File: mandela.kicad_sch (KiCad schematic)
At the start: 2 parts

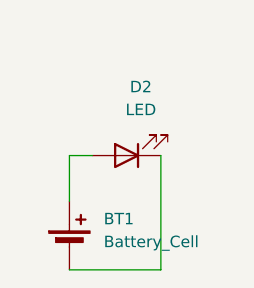
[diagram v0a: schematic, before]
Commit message: Update files
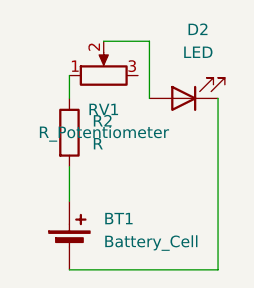
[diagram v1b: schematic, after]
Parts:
- added R2: R, no_silk:R_Axial_DIN0207_L6.3mm_D2.5mm_P7.62mm_Horizontal, symbol Device:R
- added RV1: R_Potentiometer, no_silk:Potentiometer_Vishay_T73YP_Vertical, symbol Device:R_Potentiometer
- D2: footprint LED_THT:LED_D5.0mm -> no_silk:LED_D5.0mm
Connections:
- net at BT1.1 (+): now also R2.2; no longer D2.2 (A)
- new net: D2.2 (A), RV1.2
- new net: R2.1, RV1.1
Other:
- moved on the sheet: D2
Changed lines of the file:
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@@
 	(wire
 		(pts
-			(xy 62.23 104.14) (xy 62.23 99.06)
-		)
-		(stroke
-			(width 0)
-			(type default)
-		)
-	)
-	(wire
-		(pts
-			(xy 72.39 111.76) (xy 62.23 111.76)
-		)
-		(stroke
-			(width 0)
-			(type default)
-		)
-	)
-	(wire
-		(pts
-			(xy 72.39 99.06) (xy 72.39 111.76)
-		)
-		(stroke
-			(width 0)
-			(type default)
-		)
-	)
-	(wire
-		(pts
-			(xy 62.23 99.06) (xy 64.77 99.06)
+			(xy 66.04 86.36) (xy 71.12 86.36)
+		)
+		(stroke
+			(width 0)
+			(type default)
+		)
+	)
+	(wire
+		(pts
+			(xy 62.23 100.33) (xy 62.23 104.14)
+		)
+		(stroke
+			(width 0)
+			(type default)
+		)
+	)
+	(wire
+		(pts
+			(xy 78.74 111.76) (xy 62.23 111.76)
+		)
+		(stroke
+			(width 0)
+			(type default)
+		)
+	)
+	(wire
+		(pts
+			(xy 71.12 86.36) (xy 71.12 92.71)
+		)
+		(stroke
+			(width 0)
+			(type default)
+		)
+	)
+	(wire
+		(pts
+			(xy 62.23 90.17) (xy 62.23 92.71)
+		)
+		(stroke
+			(width 0)
+			(type default)
+		)
+	)
+	(wire
+		(pts
+			(xy 78.74 92.71) (xy 78.74 111.76)
 		)
 		(stroke
@@
 	(symbol
 		(lib_id "Device:LED")
-		(at 68.58 99.06 180)
+		(at 74.93 92.71 180)
 		(unit 1)
 		(exclude_from_sim no)
@@
 		(fields_autoplaced yes)
 		(property "Reference" "D2"
-			(at 70.1675 91.44 0)
+			(at 76.5175 85.09 0)
 			(effects
 				(font
@@
 		)
 		(property "Value" "LED"
-			(at 70.1675 93.98 0)
-			(effects
-				(font
-					(size 1.27 1.27)
-				)
-			)
-		)
-		(property "Footprint" "LED_THT:LED_D5.0mm"
-			(at 68.58 99.06 0)
+			(at 76.5175 87.63 0)
+			(effects
+				(font
+					(size 1.27 1.27)
+				)
+			)
+		)
+		(property "Footprint" "no_silk:LED_D5.0mm"
+			(at 74.93 92.71 0)
 			(effects
 				(font
@@
 		)
 		(property "Datasheet" "~"
-			(at 68.58 99.06 0)
+			(at 74.93 92.71 0)
 			(effects
 				(font
@@
 		)
 		(property "Description" "Light emitting diode"
-			(at 68.58 99.06 0)
+			(at 74.93 92.71 0)
 			(effects
 				(font
@@
 		)
 		(property "Sim.Pins" "1=K 2=A"
-			(at 68.58 99.06 0)
+			(at 74.93 92.71 0)
 			(effects
 				(font
@@
 					(unit 1)
 				)
+			)
+		)
+	)
+	(symbol
+		(lib_id "Device:R")
+		(at 62.23 96.52 0)
+		(unit 1)
+		(exclude_from_sim no)
+		(in_bom yes)
+		(on_board yes)
+		(dnp no)
+		(property "Reference" "R2"
+			(at 64.77 95.2499 0)
+			(effects
+				(font
+					(size 1.27 1.27)
+				)
+				(justify left)
+			)
+		)
+		(property "Value" "R"
+			(at 64.77 97.7899 0)
+			(effects
+				(font
+					(size 1.27 1.27)
+				)
+				(justify left)
+			)
+		)
+		(property "Footprint" "no_silk:R_Axial_DIN0207_L6.3mm_D2.5mm_P7.62mm_Horizontal"
+			(at 60.452 96.52 90)
+			(effects
+				(font
+					(size 1.27 1.27)
+				)
+				(hide yes)
+			)
+		)
+		(property "Datasheet" "~"
+			(at 62.23 96.52 0)
+			(effects
+				(font
+					(size 1.27 1.27)
+				)
+				(hide yes)
+			)
+		)
+		(property "Description" "Resistor"
+			(at 62.23 96.52 0)
+			(effects
+				(font
+					(size 1.27 1.27)
+				)
+				(hide yes)
+			)
+		)
+		(pin "2"
+		)
+		(pin "1"
+		)
+		(instances
+			(project ""
+				(path "/6e1b4b5d-1e46-4a59-af59-5db0f65b54fa"
+					(reference "R2")
+					(unit 1)
+				)
+			)
+		)
+	)
+	(symbol
+		(lib_id "Device:R_Potentiometer")
+		(at 66.04 90.17 90)
+		(unit 1)
+		(exclude_from_sim no)
+		(in_bom yes)
+		(on_board yes)
+		(dnp no)
+		(fields_autoplaced yes)
+		(property "Reference" "RV1"
+			(at 66.04 93.98 90)
+			(effects
+				(font
+					(size 1.27 1.27)
+				)
+			)
+		)
+		(property "Value" "R_Potentiometer"
+			(at 66.04 96.52 90)
+			(effects
+				(font
+					(size 1.27 1.27)
+				)
+			)
+		)
+		(property "Footprint" "no_silk:Potentiometer_Vishay_T73YP_Vertical"
+			(at 66.04 90.17 0)
+			(effects
+				(font
+					(size 1.27 1.27)
+				)
+				(hide yes)
+			)
+		)
+		(property "Datasheet" "~"
+			(at 66.04 90.17 0)
+			(effects
+				(font
+					(size 1.27 1.27)
+				)
+				(hide yes)
+			)
+		)
+		(property "Description" "Potentiometer"
+			(at 66.04 90.17 0)
+			(effects
+				(font
+					(size 1.27 1.27)
+				)
+				(hide yes)
+			)
+		)
+		(pin "2"
+		)
+		(pin "3"
+		)
+		(pin "1"
+		)
+		(instances
+			(project ""
+				(path "/6e1b4b5d-1e46-4a59-af59-5db0f65b54fa"
+					(reference "RV1")
+					(unit 1)
+				)
